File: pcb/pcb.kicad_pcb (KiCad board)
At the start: 2 copper layers, 80 x 129.2 mm, 54 parts, among them J1 Conn_01x20, J2 Conn_01x20, J3 Battery, J4 Ultrasonic eyes, M1 Motor_L, M2 Motor_R, Q1 AO3401A, U1 QRE1113GR, U10 DRV8220SDG, U2 QRE1113GR, U3 QRE1113GR, U4 QRE1113GR, U5 QRE1113GR, U6 QRE1113GR, U7 QRE1113GR, U8 QRE1113GR, U9 DRV8220SDG

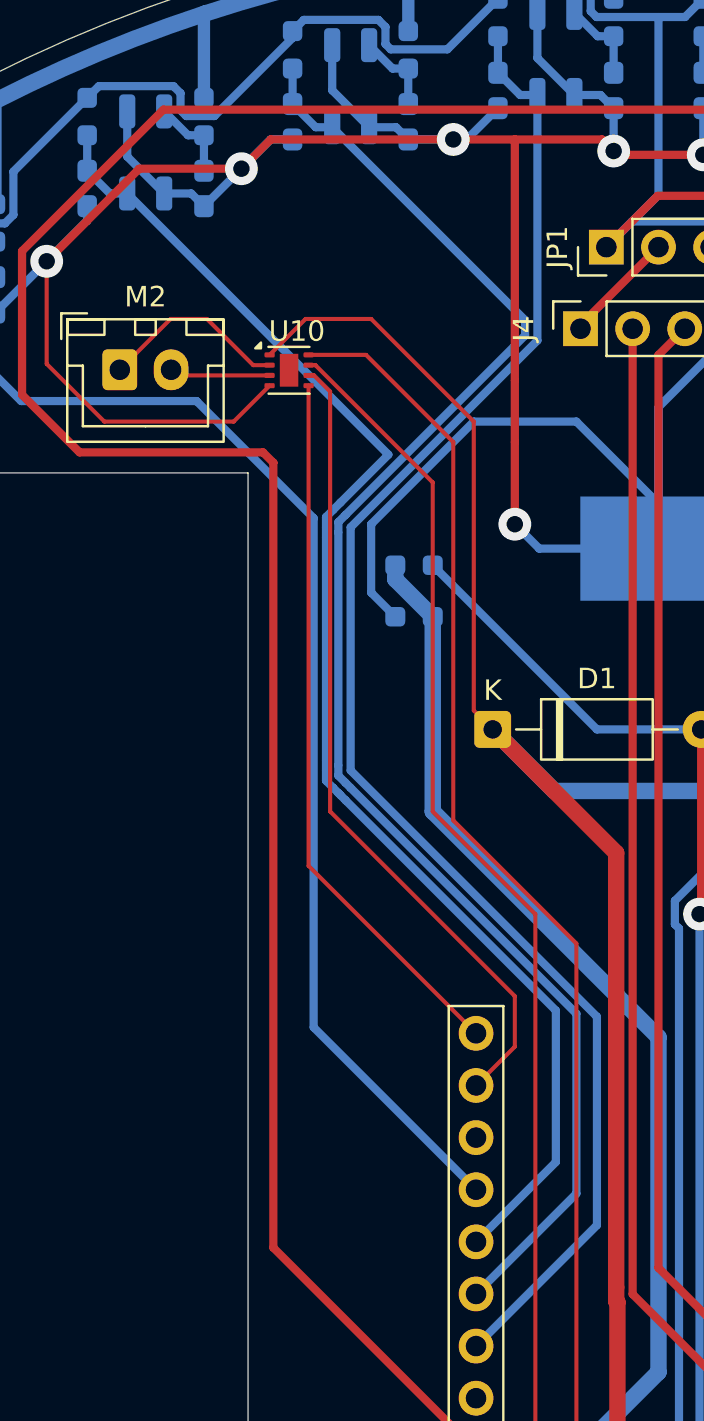
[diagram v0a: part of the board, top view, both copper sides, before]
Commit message: pcb upravená cestička
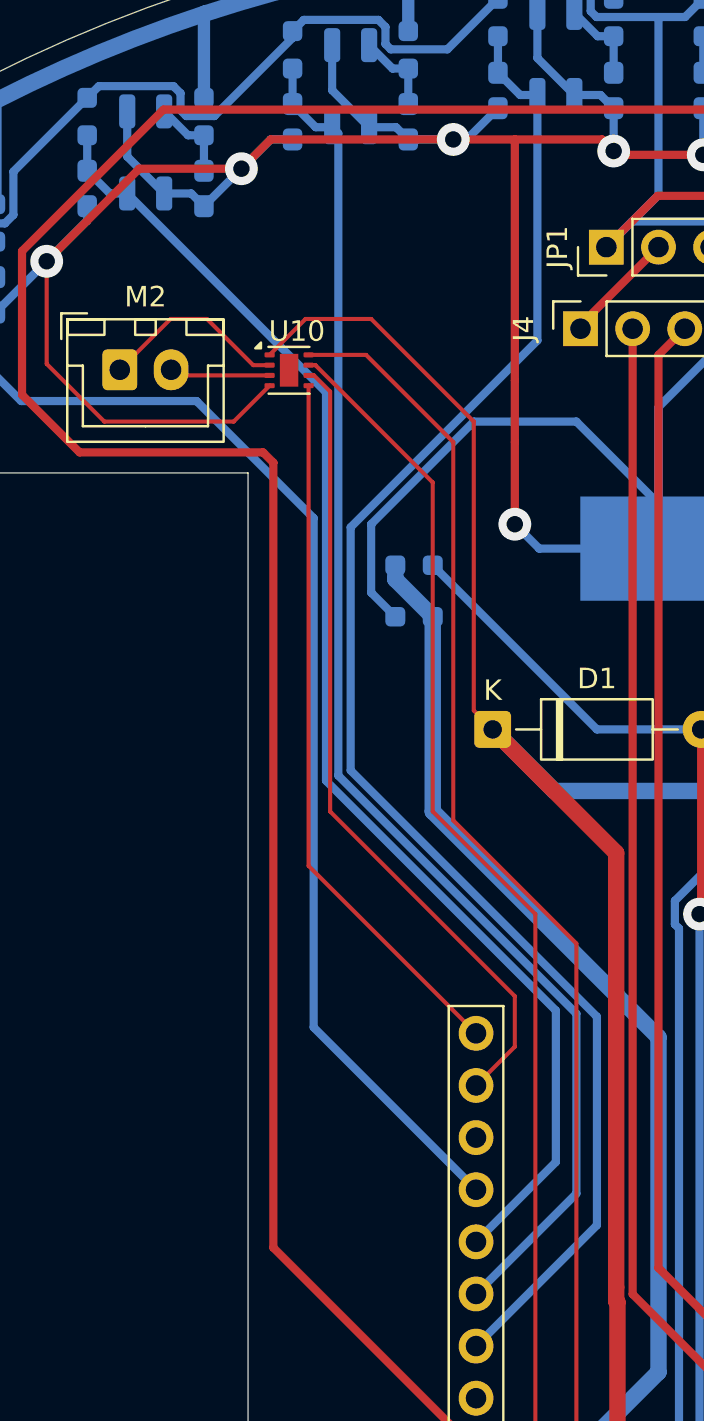
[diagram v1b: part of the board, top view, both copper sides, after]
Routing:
- net /SENSOR_2: track 75.5 -> 67.9 mm
- net /SENSOR_1: track 68.0 -> 65.5 mm
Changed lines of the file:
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@@
-	)
-	(segment
-		(start 85 96.08)
-		(end 81.11 99.97)
-		(width 0.4)
-		(layer "B.Cu")
-		(net 7)
-	)
-	(segment
-		(start 74.399 78.098884)
-		(end 74.502116 78.202)
-		(width 0.4)
-		(layer "B.Cu")
-		(net 7)
 	)
 	(segment
@@
 	)
 	(segment
-		(start 73.798 65.647942)
-		(end 73.798 76.502116)
+		(start 73.798 58.57039)
+		(end 64.1128 48.88519)
 		(width 0.4)
 		(layer "B.Cu")
@@
 	(segment
 		(start 85 88.699884)
-		(end 85 96.08)
+		(end 73.798 77.497884)
 		(width 0.4)
 		(layer "B.Cu")
@@
 	)
 	(segment
+		(start 73.798 77.497884)
+		(end 73.798 58.57039)
+		(width 0.4)
+		(layer "B.Cu")
+		(net 7)
+	)
+	(segment
 		(start 64.1128 48.88519)
 		(end 63.26809 48.88519)
@@
 	)
 	(segment
-		(start 74.502116 78.202)
-		(end 74.751058 78.450942)
-		(width 0.4)
-		(layer "B.Cu")
-		(net 7)
-	)
-	(segment
-		(start 73.798 76.502116)
-		(end 73.798 77)
-		(width 0.4)
-		(layer "B.Cu")
-		(net 7)
-	)
-	(segment
-		(start 74.150058 77.849942)
-		(end 74.399 78.098884)
-		(width 0.4)
-		(layer "B.Cu")
-		(net 7)
-	)
-	(segment
-		(start 74.751058 78.450942)
+		(start 81.11 99.97)
+		(end 85 96.08)
+		(width 0.4)
+		(layer "B.Cu")
+		(net 7)
+	)
+	(segment
+		(start 85 96.08)
 		(end 85 88.699884)
-		(width 0.4)
-		(layer "B.Cu")
-		(net 7)
-	)
-	(segment
-		(start 73.798 64.652174)
-		(end 73.798 65.150058)
-		(width 0.4)
-		(layer "B.Cu")
-		(net 7)
-	)
-	(segment
-		(start 74.150058 64.300116)
-		(end 73.798 64.652174)
-		(width 0.4)
-		(layer "B.Cu")
-		(net 7)
-	)
-	(segment
-		(start 73.798 77)
-		(end 73.798 77.497884)
-		(width 0.4)
-		(layer "B.Cu")
-		(net 7)
-	)
-	(segment
-		(start 76.838892 61.611282)
-		(end 74.502116 63.948058)
-		(width 0.4)
-		(layer "B.Cu")
-		(net 7)
-	)
-	(segment
-		(start 73.798 65.150058)
-		(end 73.798 65.647942)
-		(width 0.4)
-		(layer "B.Cu")
-		(net 7)
-	)
-	(segment
-		(start 73.798 77.497884)
-		(end 74.150058 77.849942)
-		(width 0.4)
-		(layer "B.Cu")
-		(net 7)
-	)
-	(segment
-		(start 64.1128 48.88519)
-		(end 76.838892 61.611282)
-		(width 0.4)
-		(layer "B.Cu")
-		(net 7)
-	)
-	(segment
-		(start 74.502116 63.948058)
-		(end 74.150058 64.300116)
 		(width 0.4)
 		(layer "B.Cu")
@@
 	)
 	(segment
-		(start 83.499 55.055551)
-		(end 83.499 55.801116)
-		(width 0.4)
-		(layer "B.Cu")
-		(net 12)
-	)
-	(segment
 		(start 73.298251 45.656551)
 		(end 72.1692 44.5275)
@@
 	)
 	(segment
-		(start 74.751058 64.549058)
-		(end 74.399 64.901116)
-		(width 0.4)
-		(layer "B.Cu")
-		(net 12)
-	)
-	(segment
-		(start 74.399 65.399)
-		(end 74.399 76.751058)
-		(width 0.4)
-		(layer "B.Cu")
-		(net 12)
-	)
-	(segment
-		(start 74.751058 77.601)
-		(end 75 77.849942)
-		(width 0.4)
-		(layer "B.Cu")
-		(net 12)
-	)
-	(segment
-		(start 74.399 76.751058)
-		(end 74.399 77.248942)
+		(start 74.399 77.248942)
+		(end 74.399 45.955551)
+		(width 0.4)
+		(layer "B.Cu")
+		(net 12)
+	)
+	(segment
+		(start 81.11 102.51)
+		(end 86 97.62)
 		(width 0.4)
 		(layer "B.Cu")
@@
 	(segment
 		(start 86 97.62)
-		(end 81.11 102.51)
-		(width 0.4)
-		(layer "B.Cu")
-		(net 12)
-	)
-	(segment
-		(start 74.399 64.901116)
-		(end 74.399 65.399)
+		(end 86 88.849942)
 		(width 0.4)
 		(layer "B.Cu")
@@
 	)
 	(segment
-		(start 75 77.849942)
-		(end 86 88.849942)
-		(width 0.4)
-		(layer "B.Cu")
-		(net 12)
-	)
-	(segment
 		(start 72.1692 42.7973)
 		(end 72.1692 44.5275)
@@
 	)
 	(segment
+		(start 74.399 45.955551)
+		(end 74.1 45.656551)
+		(width 0.4)
+		(layer "B.Cu")
+		(net 12)
+	)
+	(segment
 		(start 86 88.849942)
-		(end 86 97.62)
-		(width 0.4)
-		(layer "B.Cu")
-		(net 12)
-	)
-	(segment
-		(start 83.499 55.801116)
-		(end 74.751058 64.549058)
-		(width 0.4)
-		(layer "B.Cu")
-		(net 12)
-	)
-	(segment
-		(start 74.399 77.248942)
-		(end 74.751058 77.601)
-		(width 0.4)
-		(layer "B.Cu")
-		(net 12)
-	)
-	(segment
-		(start 74.1 45.656551)
-		(end 83.499 55.055551)
-		(width 0.4)
-		(layer "B.Cu")
+		(end 74.399 77.248942)
+		(width 0.4)
+		(layer "B.Cu")
